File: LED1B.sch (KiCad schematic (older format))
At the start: 18 parts

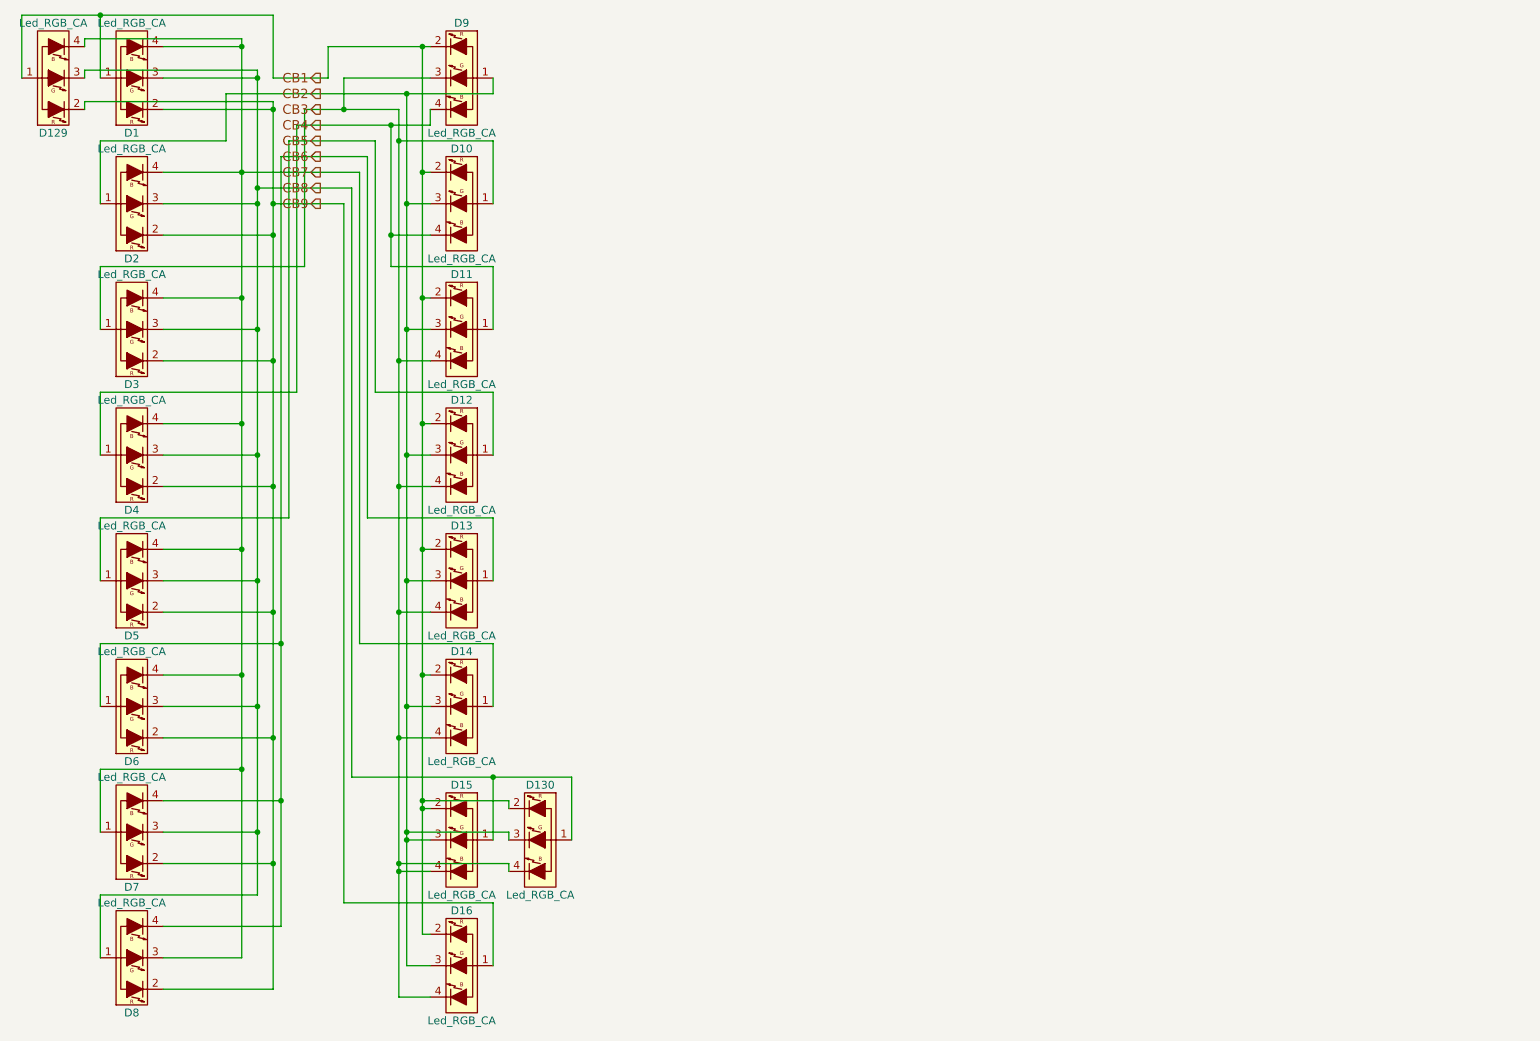
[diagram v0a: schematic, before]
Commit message: Clean up LED-Schematics
Luckily I didn't make any mistakes in the first run.
(Unless I made the same Mistake twice)
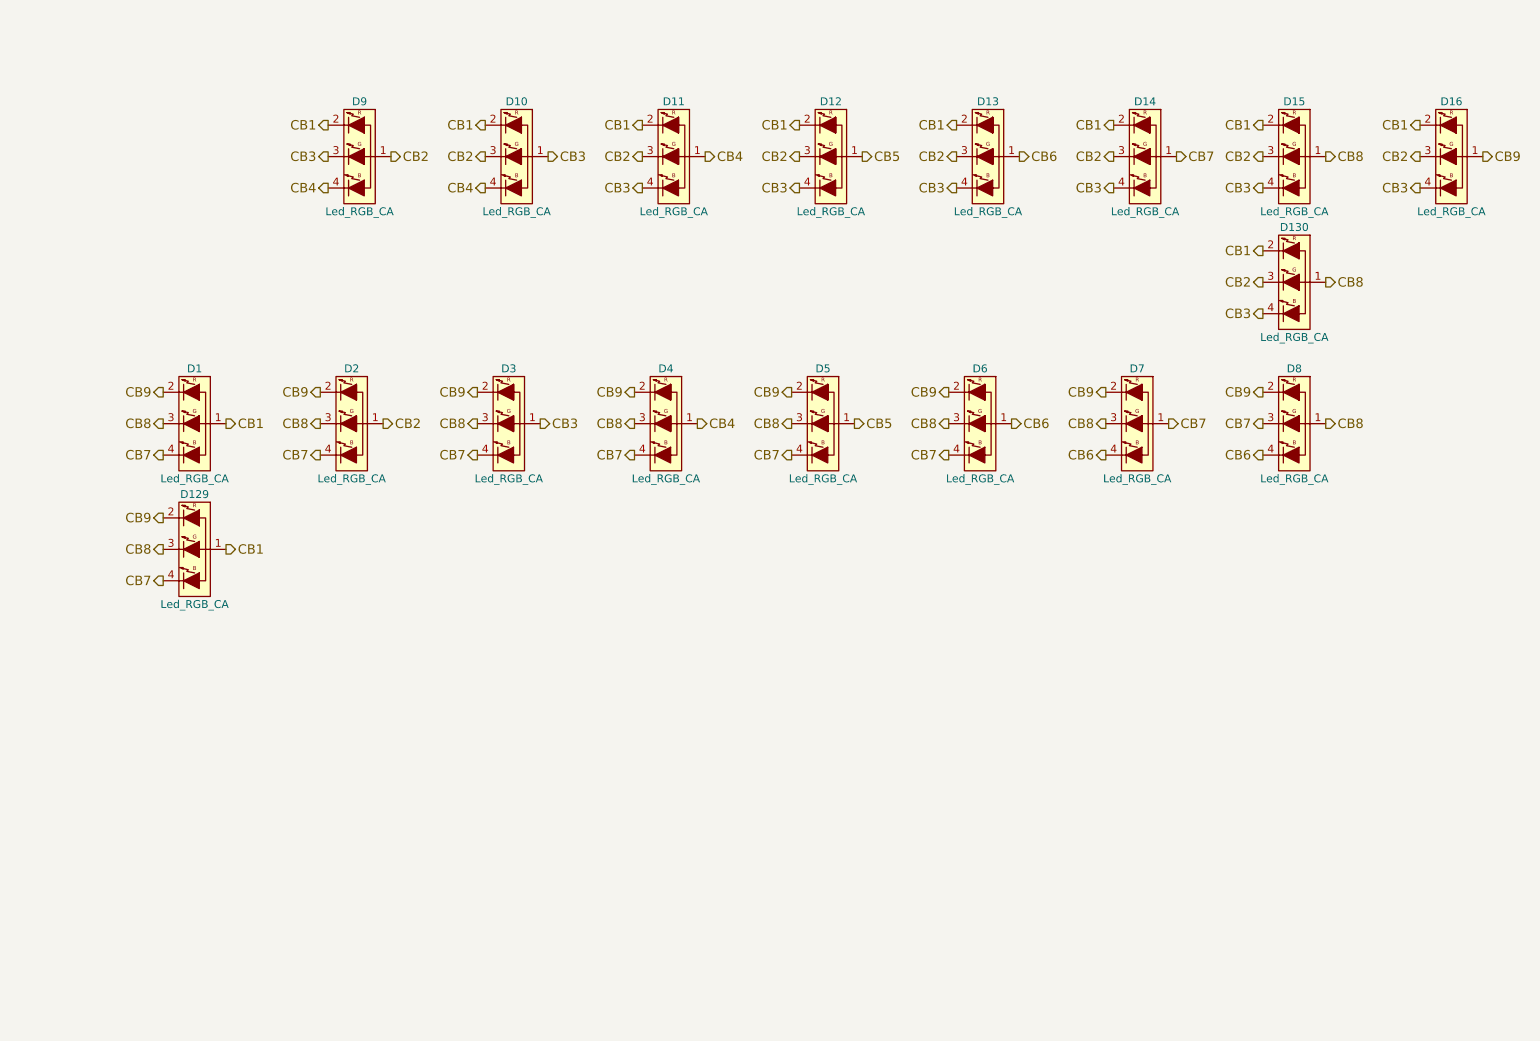
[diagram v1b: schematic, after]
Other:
- moved on the sheet: D1, D10, D11, D12, D129, D13, D130, D14, D15, D16, D2, D3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
